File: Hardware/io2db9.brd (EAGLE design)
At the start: 95.1 x 31.2 mm, 22 parts

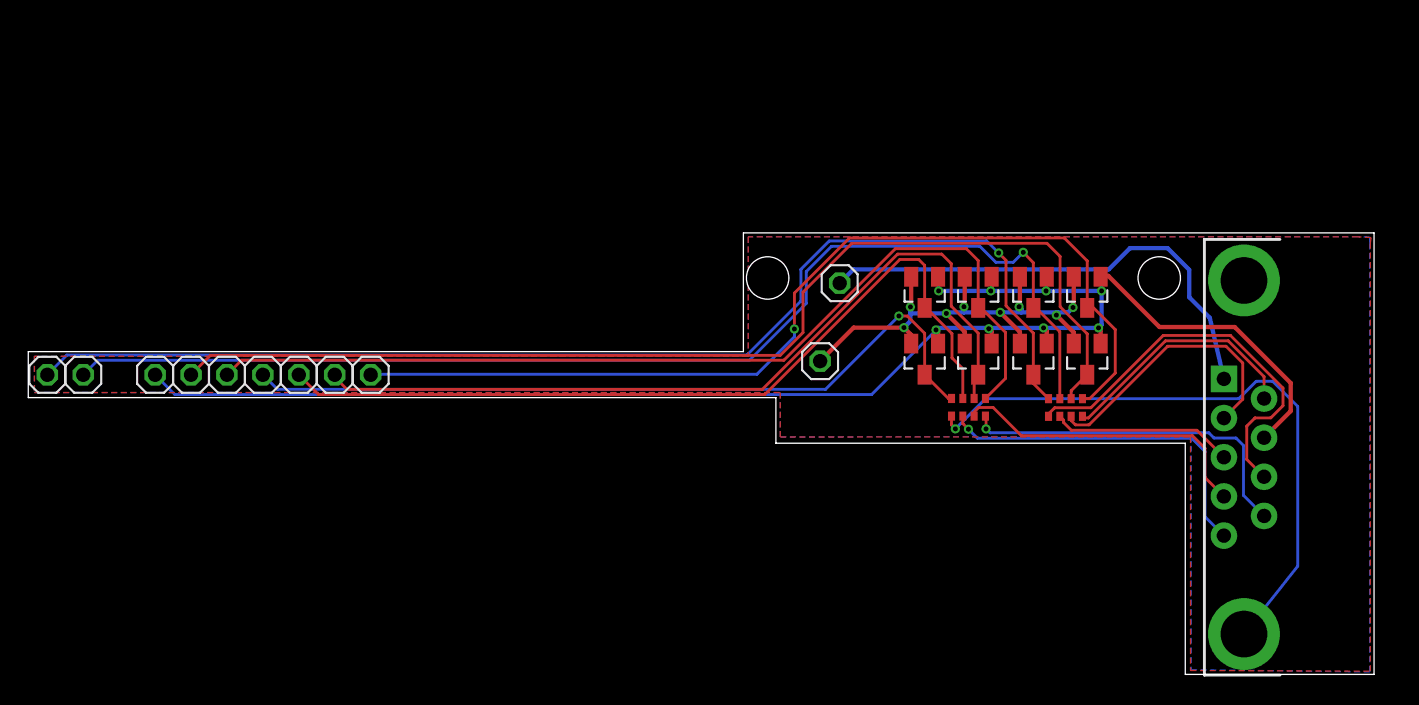
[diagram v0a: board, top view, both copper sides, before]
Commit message: updated
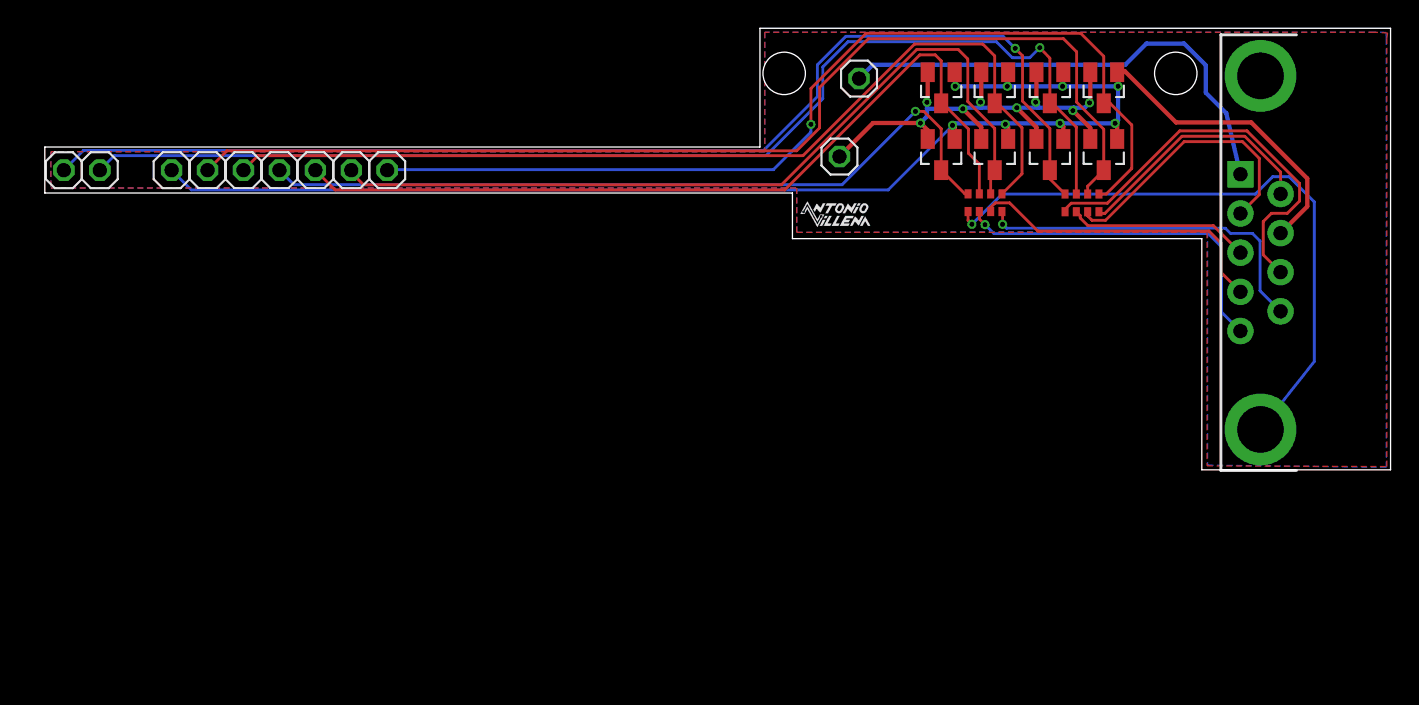
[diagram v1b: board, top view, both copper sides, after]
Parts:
- moved JP1 14.5 mm to (56.8, 22.4)
- moved JP3 14.5 mm to (55.4, 16.9)
- moved D2 14.5 mm to (70.3, 17.0)
- moved D4 14.5 mm to (62.6, 17.0)
- moved D6 14.5 mm to (74.1, 17.0)
- moved D7 14.5 mm to (66.4, 17.0)
- moved D1 14.5 mm to (70.3, 21.7)
- moved D3 14.5 mm to (62.6, 21.7)
- moved D5 14.5 mm to (66.4, 21.7)
- moved D8 14.5 mm to (74.1, 21.7)
- moved J1 14.5 mm to (85.2, 10.1)
- moved JP10 14.5 mm to (10.8, 15.9)
- moved JP11 14.5 mm to (13.3, 15.9)
- moved JP12 14.5 mm to (15.8, 15.9)
- moved JP13 14.5 mm to (18.4, 15.9)
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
